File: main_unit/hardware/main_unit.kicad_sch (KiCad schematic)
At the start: 14 parts, among them SW1 SW_SPST, U1 STM32H753ZIT6, Y1 ABM8G-25.000MHZ-18-D2Y-T, Y2 SC32S-7PF20PPM

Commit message: main_unit/hardware: Fix STM32 to use LQFP-144 package instead of LQFP-100
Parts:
- U1: footprint Package_QFP:LQFP-100_14x14mm_P0.5mm -> Package_QFP:LQFP-144_20x20mm_P0.5mm
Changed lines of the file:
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@@
 			)
 		)
-		(property "Footprint" "Package_QFP:LQFP-100_14x14mm_P0.5mm"
+		(property "Footprint" "Package_QFP:LQFP-144_20x20mm_P0.5mm"
 			(at 234.95 120.65 0)
 			(effects

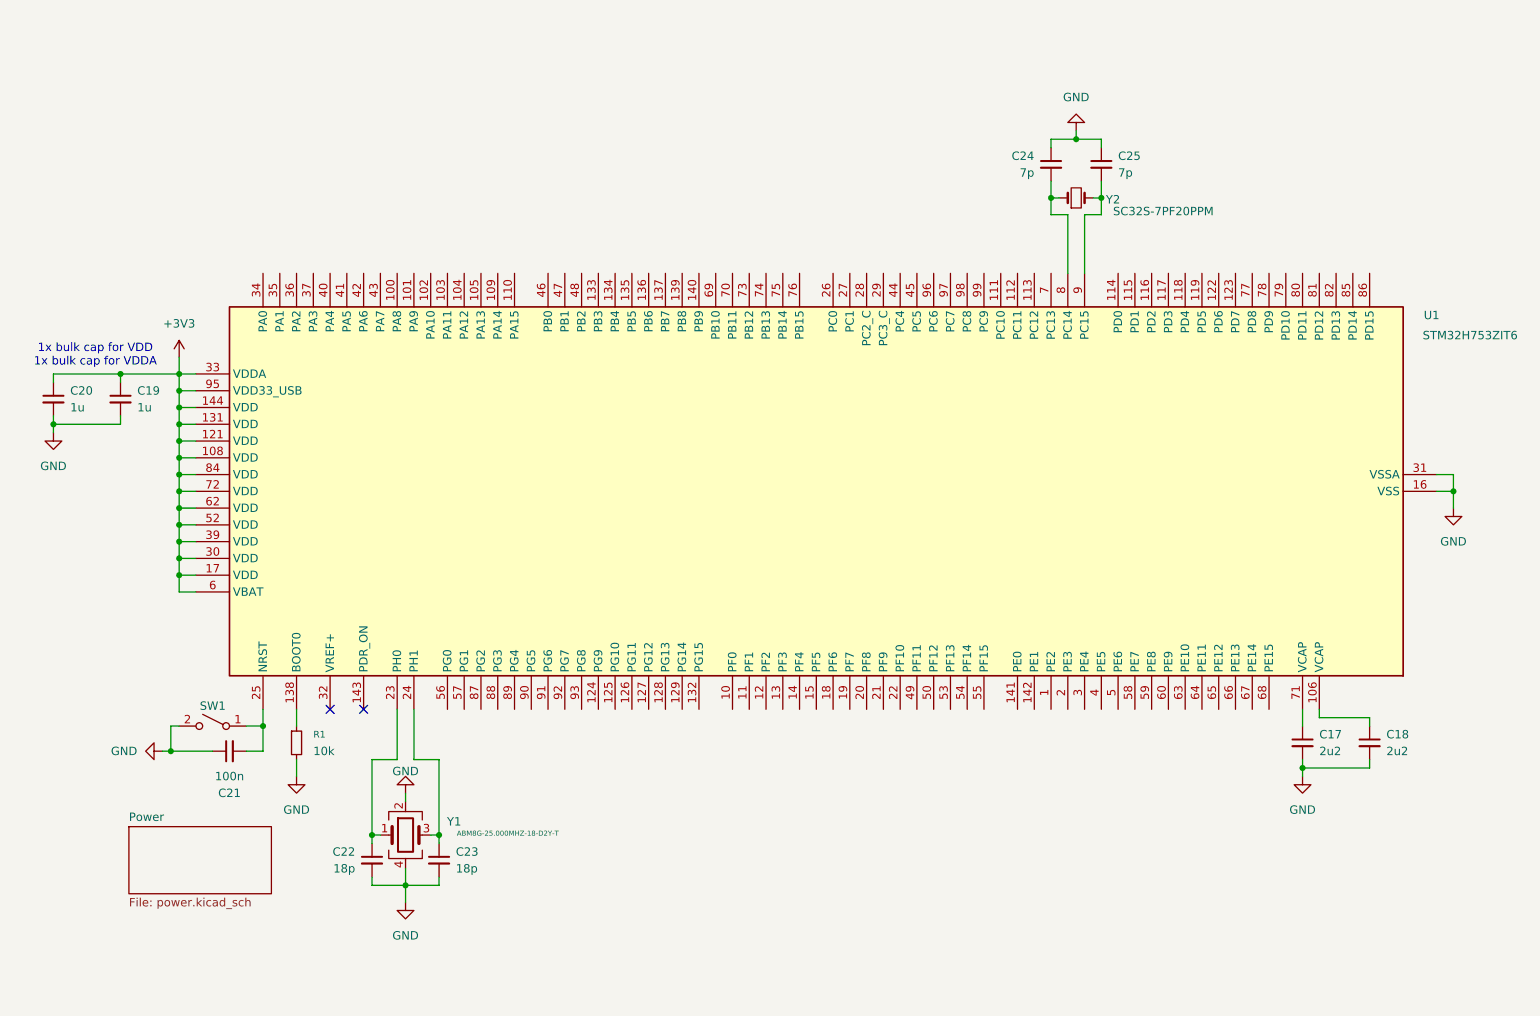
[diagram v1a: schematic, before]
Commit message: main_unit/hardware: Assign all pins for STM32
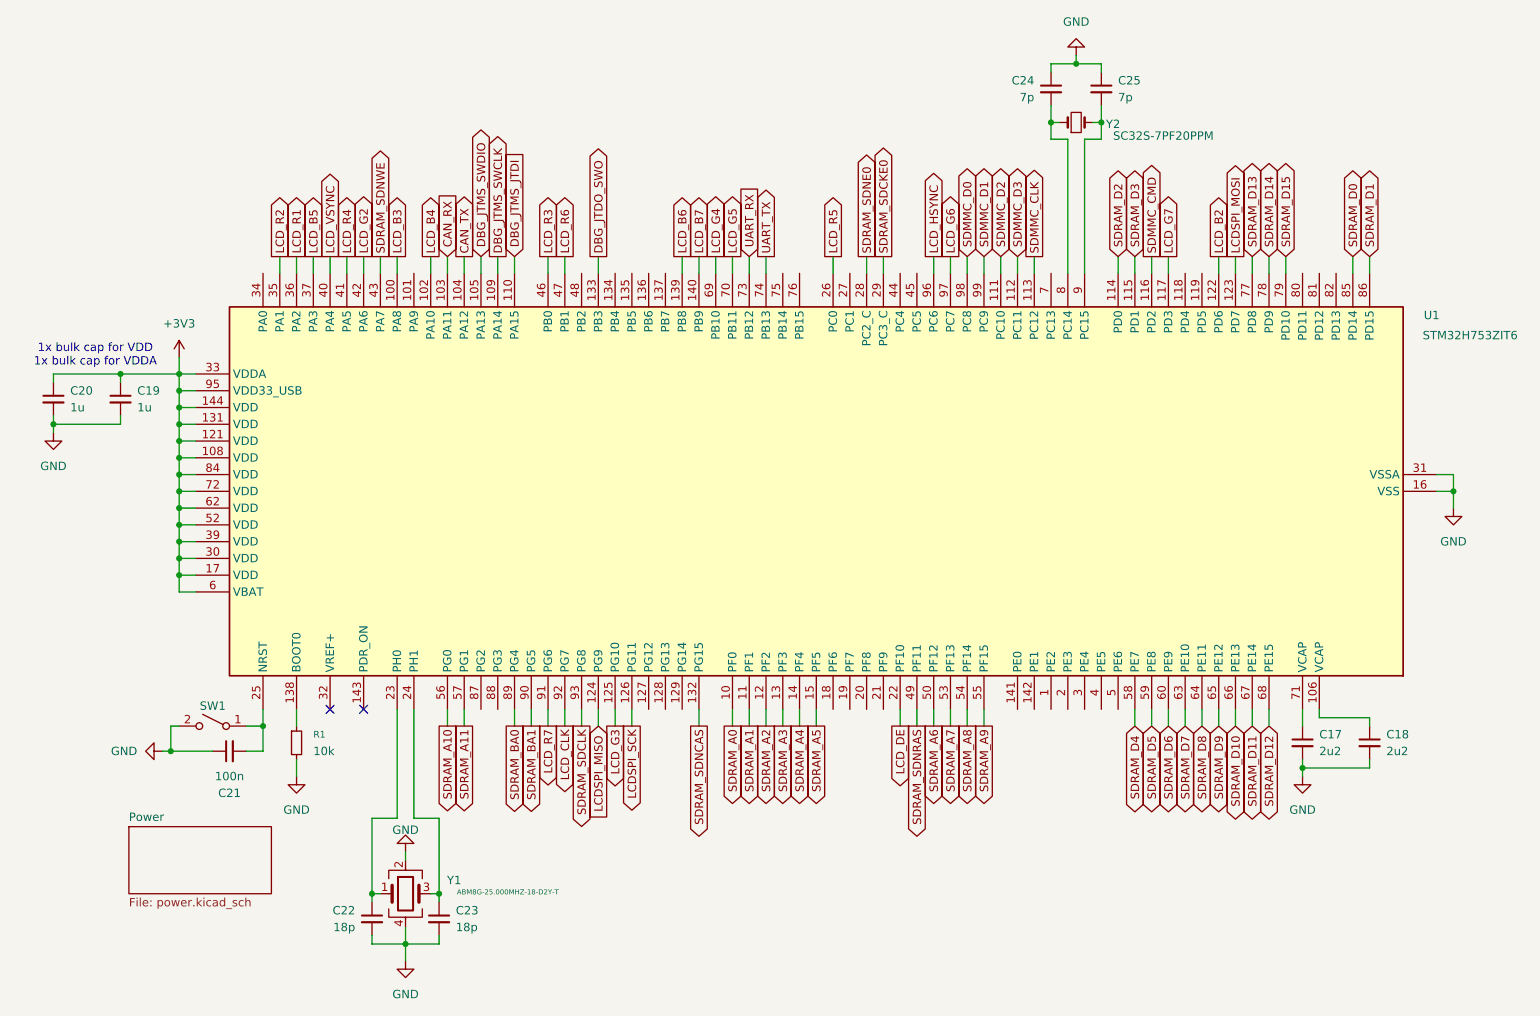
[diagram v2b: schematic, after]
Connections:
- net SDRAM_A0: now reaches U1.10 (PF0)
- net LCD_B3: now reaches U1.100 (PA8)
- net LCD_B4: now reaches U1.102 (PA10)
- net CAN_RX: now reaches U1.103 (PA11)
- net CAN_TX: now reaches U1.104 (PA12)
- net DBG_JTMS_SWDIO: now reaches U1.105 (PA13)
- net DBG_JTMS_SWCLK: now reaches U1.109 (PA14)
- net SDRAM_A1: now reaches U1.11 (PF1)
- net DBG_JTMS_JTDI: now reaches U1.110 (PA15)
- net SDMMC_D2: now reaches U1.111 (PC10)
- net SDMMC_D3: now reaches U1.112 (PC11)
- net SDMMC_CLK: now reaches U1.113 (PC12)
- net SDRAM_D2: now reaches U1.114 (PD0)
- net SDRAM_D3: now reaches U1.115 (PD1)
- net SDMMC_CMD: now reaches U1.116 (PD2)
- net LCD_G7: now reaches U1.117 (PD3)
- net SDRAM_A2: now reaches U1.12 (PF2)
- net LCD_B2: now reaches U1.122 (PD6)
- net LCDSPI_MOSI: now reaches U1.123 (PD7)
- net LCDSPI_MISO: now reaches U1.124 (PG9)
- net LCD_G3: now reaches U1.125 (PG10)
- net LCDSPI_SCK: now reaches U1.126 (PG11)
- net SDRAM_A3: now reaches U1.13 (PF3)
- net SDRAM_SDNCAS: now reaches U1.132 (PG15)
- net DBG_JTDO_SWO: now reaches U1.133 (PB3)
- net LCD_B6: now reaches U1.139 (PB8)
- net SDRAM_A4: now reaches U1.14 (PF4)
- net LCD_B7: now reaches U1.140 (PB9)
- net SDRAM_A5: now reaches U1.15 (PF5)
- net LCD_DE: now reaches U1.22 (PF10)
- net LCD_R5: now reaches U1.26 (PC0)
- net SDRAM_SDNE0: now reaches U1.28 (PC2_C)
- net SDRAM_SDCKE0: now reaches U1.29 (PC3_C)
- net LCD_R2: now reaches U1.35 (PA1)
- net LCD_R1: now reaches U1.36 (PA2)
- net LCD_B5: now reaches U1.37 (PA3)
- net LCD_VSYNC: now reaches U1.40 (PA4)
- net LCD_R4: now reaches U1.41 (PA5)
- net LCD_G2: now reaches U1.42 (PA6)
- net SDRAM_SDNWE: now reaches U1.43 (PA7)
- net LCD_R3: now reaches U1.46 (PB0)
- net LCD_R6: now reaches U1.47 (PB1)
- net SDRAM_SDNRAS: now reaches U1.49 (PF11)
- net SDRAM_A6: now reaches U1.50 (PF12)
- net SDRAM_A7: now reaches U1.53 (PF13)
- net SDRAM_A8: now reaches U1.54 (PF14)
- net SDRAM_A9: now reaches U1.55 (PF15)
- net SDRAM_A10: now reaches U1.56 (PG0)
- net SDRAM_A11: now reaches U1.57 (PG1)
- net SDRAM_D4: now reaches U1.58 (PE7)
- net SDRAM_D5: now reaches U1.59 (PE8)
- net SDRAM_D6: now reaches U1.60 (PE9)
- net SDRAM_D7: now reaches U1.63 (PE10)
- net SDRAM_D8: now reaches U1.64 (PE11)
- net SDRAM_D9: now reaches U1.65 (PE12)
- net SDRAM_D10: now reaches U1.66 (PE13)
- net SDRAM_D11: now reaches U1.67 (PE14)
- net SDRAM_D12: now reaches U1.68 (PE15)
- net LCD_G4: now reaches U1.69 (PB10)
- net LCD_G5: now reaches U1.70 (PB11)
- net UART_RX: now reaches U1.73 (PB12)
- net UART_TX: now reaches U1.74 (PB13)
- net SDRAM_D13: now reaches U1.77 (PD8)
- net SDRAM_D14: now reaches U1.78 (PD9)
- net SDRAM_D15: now reaches U1.79 (PD10)
- net SDRAM_D0: now reaches U1.85 (PD14)
- net SDRAM_D1: now reaches U1.86 (PD15)
- net SDRAM_BA0: now reaches U1.89 (PG4)
- net SDRAM_BA1: now reaches U1.90 (PG5)
- net LCD_R7: now reaches U1.91 (PG6)
- net LCD_CLK: now reaches U1.92 (PG7)
- net SDRAM_SDCLK: now reaches U1.93 (PG8)
- net LCD_HSYNC: now reaches U1.96 (PC6)
- net LCD_G6: now reaches U1.97 (PC7)
- net SDMMC_D0: now reaches U1.98 (PC8)
- net SDMMC_D1: now reaches U1.99 (PC9)
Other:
- moved on the sheet: C22, C23, C24, C25, Y1, Y2
